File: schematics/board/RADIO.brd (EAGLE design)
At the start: 29 x 49 mm, 2 parts

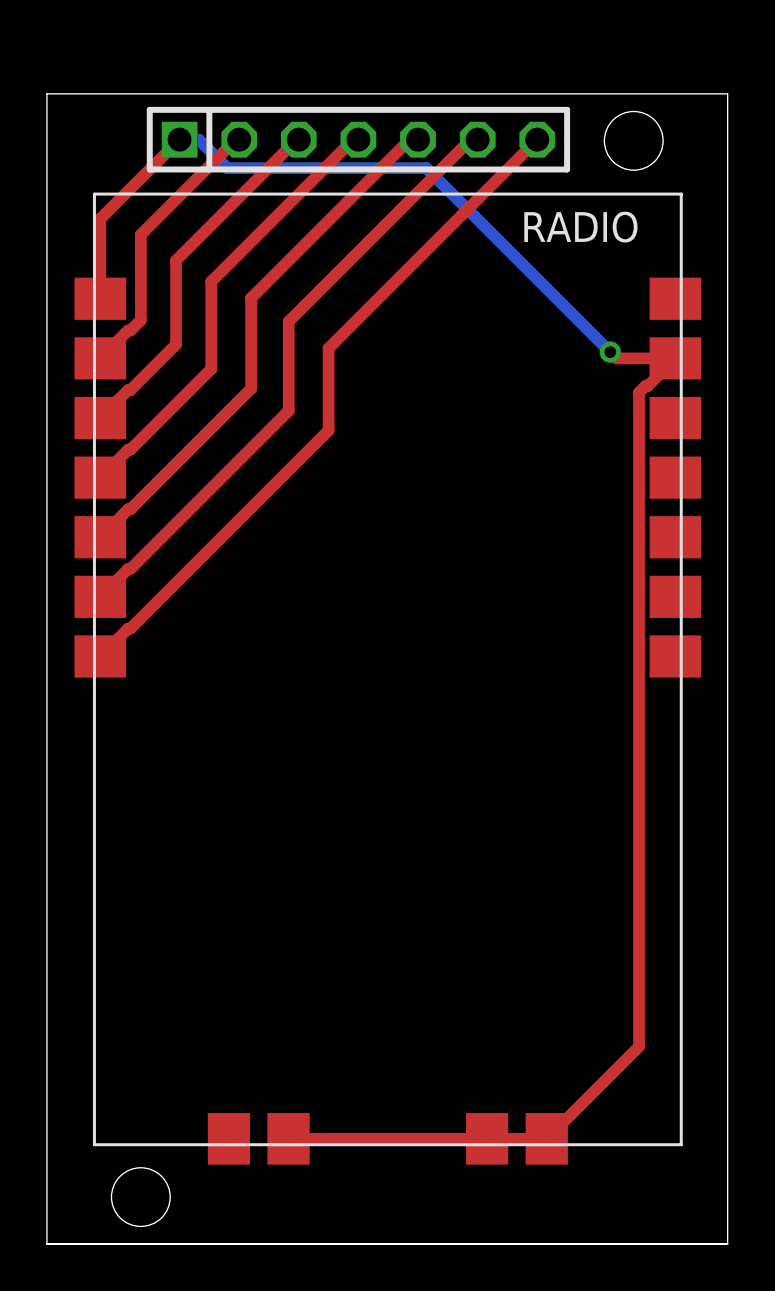
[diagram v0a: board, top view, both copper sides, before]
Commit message: Платы подготовлены для Резонита
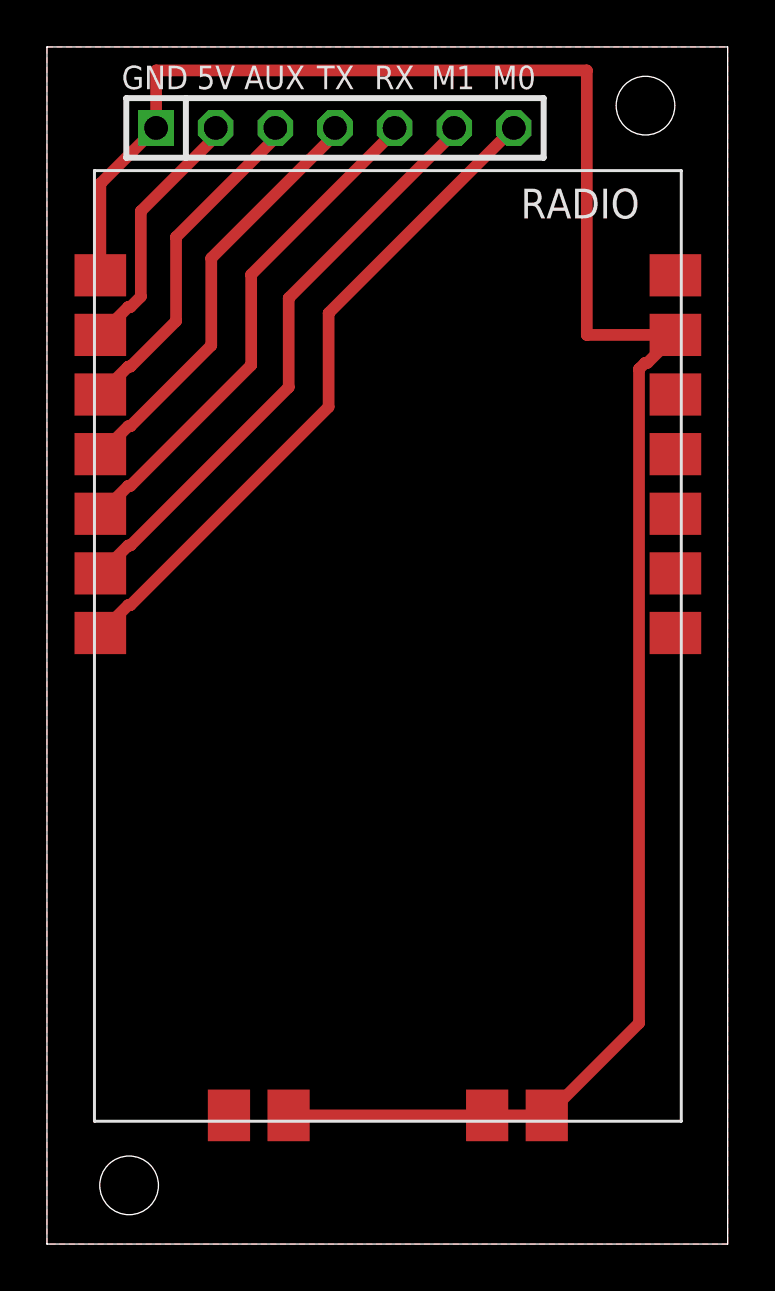
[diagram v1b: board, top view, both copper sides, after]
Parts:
- moved JP1 1.12 mm to (12.3, 47.5)
- moved RADIO 1.00 mm to (27.0, 5.23)
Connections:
- net N$1 renamed GND
- net N$2 renamed 5V
- net N$3 renamed AUX
- net N$4 renamed TXD
- net N$5 renamed RXD
- net N$6 renamed M1
- net N$7 renamed M0
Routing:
- net GND: track 79.7 -> 89.7 mm, vias 1 -> 0
- net RXD: track 22.8 -> 21.7 mm
- net M1: track 26.4 -> 25.3 mm
- net TXD: track 19.1 -> 18.1 mm
- net 5V: track 11.9 -> 10.9 mm
- net AUX: track 15.5 -> 14.5 mm
- net M0: track 29.8 -> 28.9 mm
- added copper zone on layer 1, net GND
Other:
- board size 29 x 49 mm -> 29 x 51 mm
- board text added: "5V"
- board text added: "AUX"
- board text added: "GND"
- board text added: "M0"
- board text added: "M1"
- board text added: "RX"
- board text added: "TX"
